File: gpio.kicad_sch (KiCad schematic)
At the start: 19 parts, among them J10 GPIO0, J13 GPIO1, J16 SCOOP1, J17 SCOOP2, J18 ACTUATOR, J19 DRILL, J20 SERVO5, J21 SERVO6, J22 SERVO7, J23 SERVO8, J5 MOIST, J6 TEMP, J7 POT3, J9 GPIO, U15 74HCT244, U8 PCA9555PWR

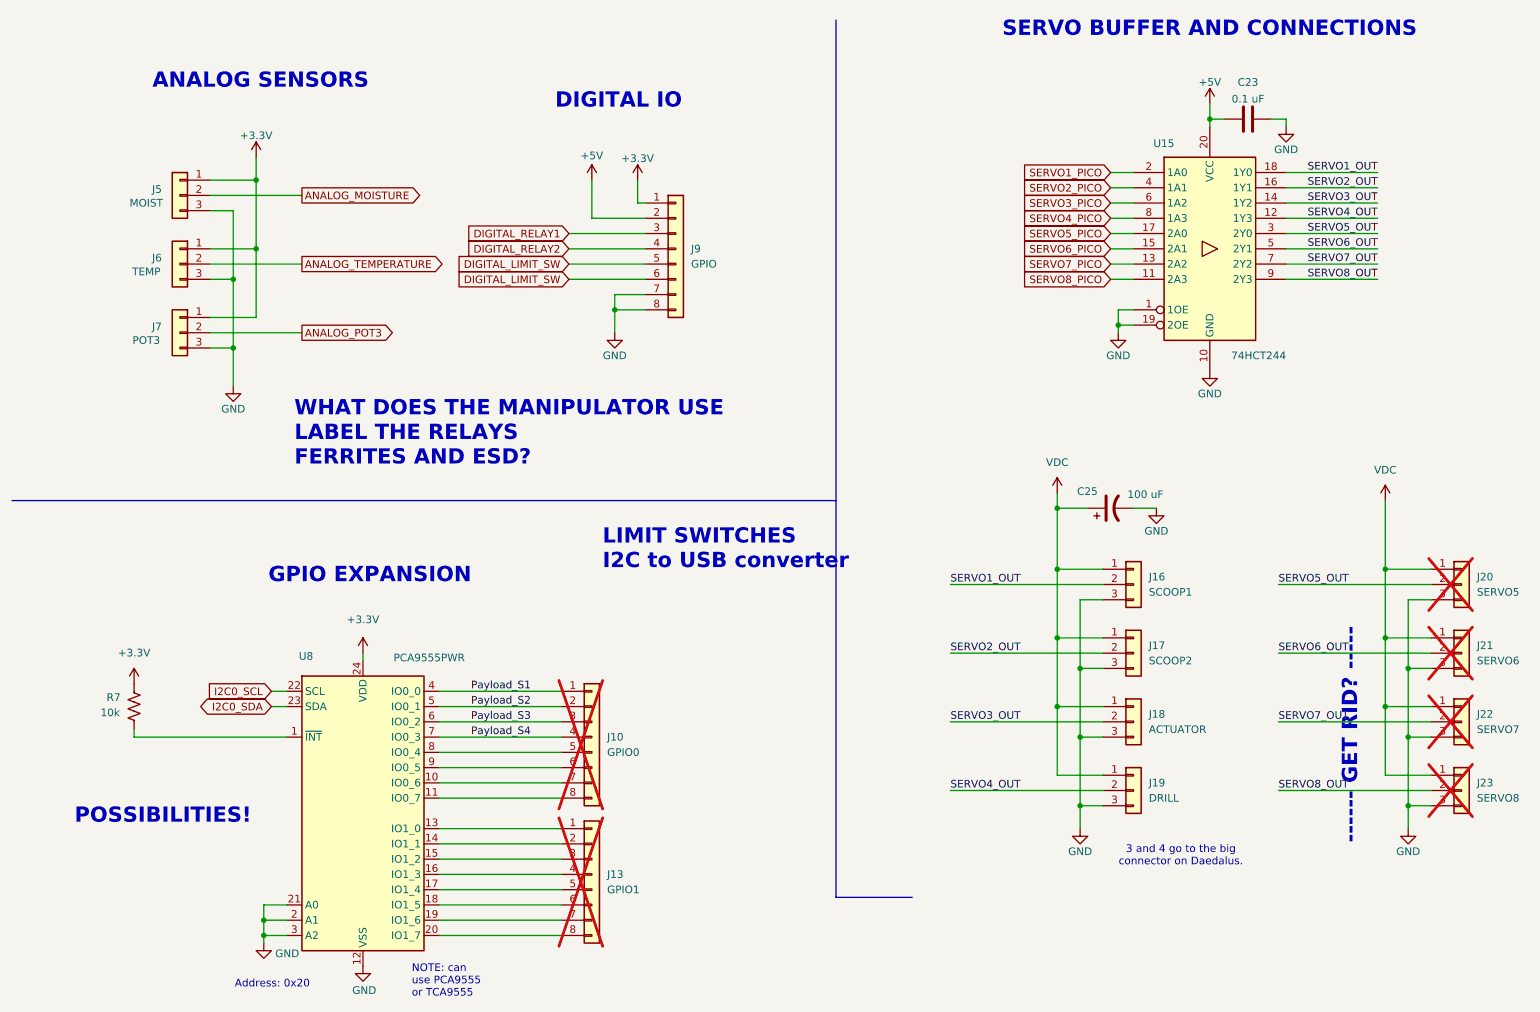
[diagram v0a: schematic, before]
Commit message: major rework again after the meeting
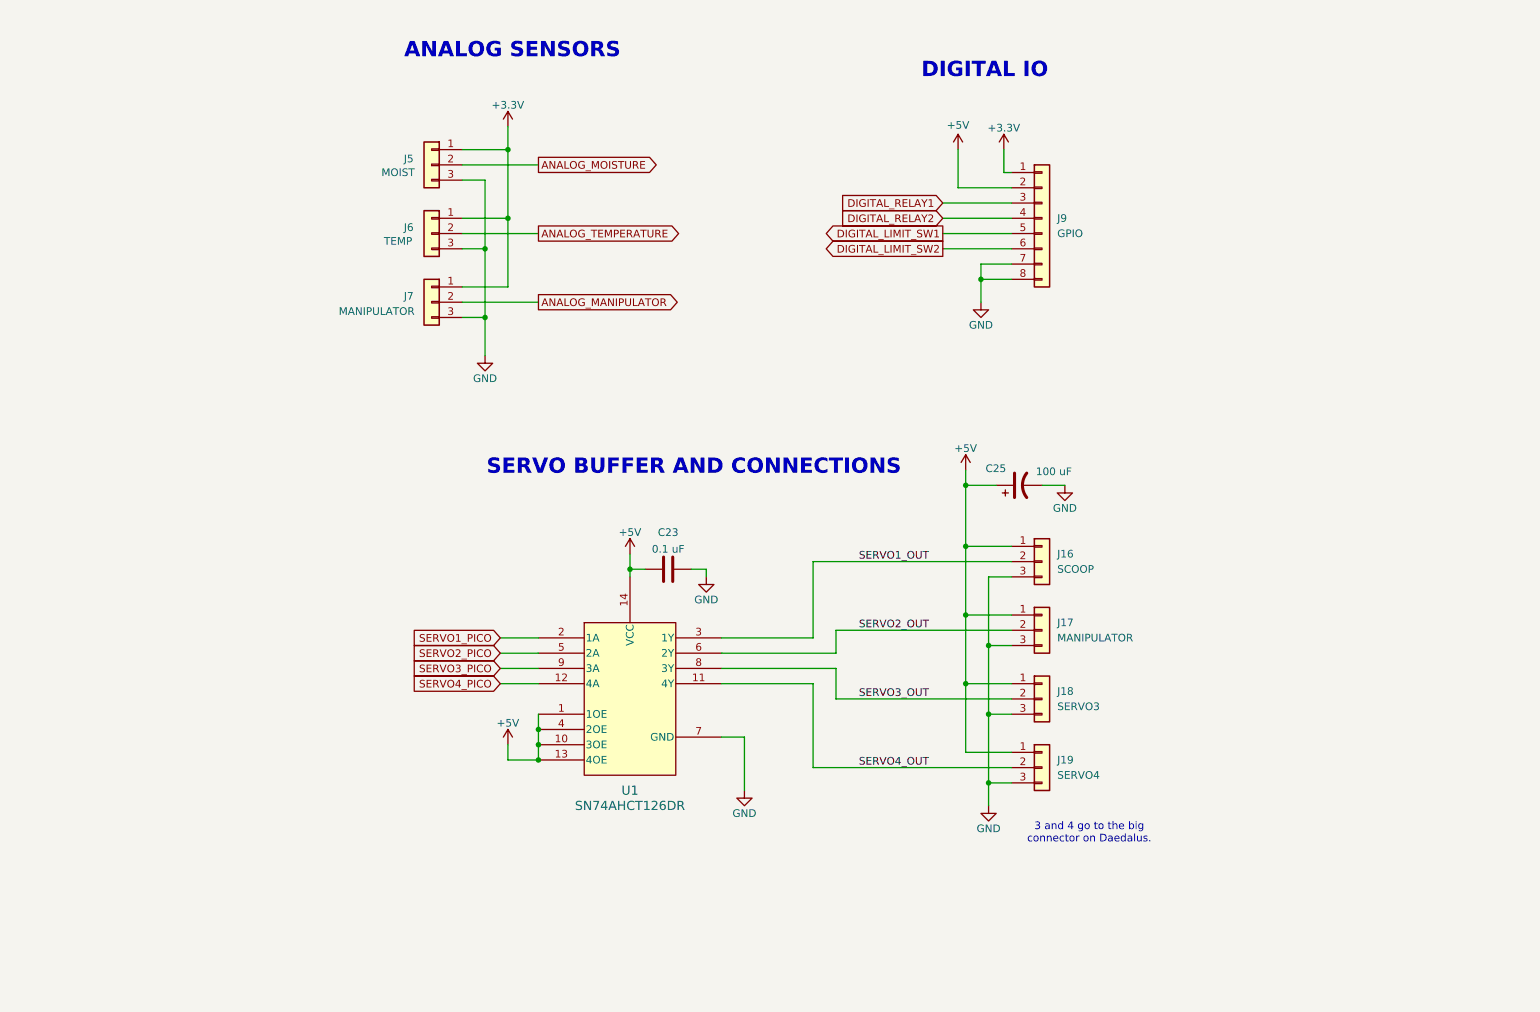
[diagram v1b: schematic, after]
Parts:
- removed J10: GPIO0, Connector_Molex:Molex_PicoBlade_53047-0810_1x08_P1.25mm_Vertical, symbol Connector_Generic:Conn_01x08
- removed J13: GPIO1, Connector_Molex:Molex_PicoBlade_53047-0810_1x08_P1.25mm_Vertical, symbol Connector_Generic:Conn_01x08
- removed J20: SERVO5, Connector_Molex:Molex_PicoBlade_53047-0310_1x03_P1.25mm_Vertical, symbol Connector_Generic:Conn_01x03
- removed J21: SERVO6, Connector_Molex:Molex_PicoBlade_53047-0310_1x03_P1.25mm_Vertical, symbol Connector_Generic:Conn_01x03
- removed J22: SERVO7, Connector_Molex:Molex_PicoBlade_53047-0310_1x03_P1.25mm_Vertical, symbol Connector_Generic:Conn_01x03
- removed J23: SERVO8, Connector_Molex:Molex_PicoBlade_53047-0310_1x03_P1.25mm_Vertical, symbol Connector_Generic:Conn_01x03
- removed R7: 10k, Resistor_SMD:R_0805_2012Metric_Pad1.20x1.40mm_HandSolder, symbol Device:R_US
- removed U15: 74HCT244, Package_SO:SO-20_12.8x7.5mm_P1.27mm, symbol 74xx:74HCT244
- removed U8: PCA9555PWR, Package_SO:TSSOP-24_4.4x7.8mm_P0.65mm, symbol Interface_Expansion:PCA9555DB
- added U1: SN74AHCT126DR, Package_SO:SOIC-14_3.9x8.7mm_P1.27mm, symbol symbols:SN74AHCT126DR
- J16: value SCOOP1 -> SCOOP
- J17: value SCOOP2 -> MANIPULATOR
- J18: value ACTUATOR -> SERVO3
- J19: value DRILL -> SERVO4
- J7: value POT3 -> MANIPULATOR
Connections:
- net VDC is gone; now on net +5V: C25.1, J16.1 (Pin_1), J17.1 (Pin_1), J18.1 (Pin_1), J19.1 (Pin_1)
- net +5V: now also U1.1 (1OE), U1.10 (3OE), U1.13 (4OE), U1.14 (VCC), U1.4 (2OE)
- net GND: now also U1.7 (GND)
- net SERVO1_OUT: now also U1.3 (1Y)
- net SERVO1_PICO: now also U1.2 (1A)
- net SERVO2_OUT: now also U1.6 (2Y)
- net SERVO2_PICO: now also U1.5 (2A)
- net SERVO3_OUT: now also U1.8 (3Y)
- net SERVO3_PICO: now also U1.9 (3A)
- net SERVO4_OUT: now also U1.11 (4Y)
- net SERVO4_PICO: now also U1.12 (4A)
- net ANALOG_POT3 renamed ANALOG_MANIPULATOR
- net DIGITAL_LIMIT_SW renamed DIGITAL_LIMIT_SW1
- net DIGITAL_LIMIT_SW1: no longer J9.6 (Pin_6)
- new net DIGITAL_LIMIT_SW2: J9.6 (Pin_6)
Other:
- note removed: "------ GET RID? -----"
- note removed: "Address: 0x20"
- note removed: "GPIO EXPANSION"
- note removed: "LIMIT SWITCHES I2C to USB converter"
- note removed: "NOTE: can use PCA9555 or TCA9555"
- note removed: "POSSIBILITIES!"
- note removed: "WHAT DOES THE MANIPULATOR USE LABEL THE RELAYS FERRITES AND ESD?"
- moved on the sheet: C23, C25, J16, J17, J18, J19, J5, J6, J7, J9
